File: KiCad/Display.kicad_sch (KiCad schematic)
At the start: 36 parts, among them J1 DC, J2 I/O, J3 USB-C, U1 ESP32-PICO-MINI-02, U2 L96-M33, U3 FT231XQ, U4 LMR16006+FB, U5 QR

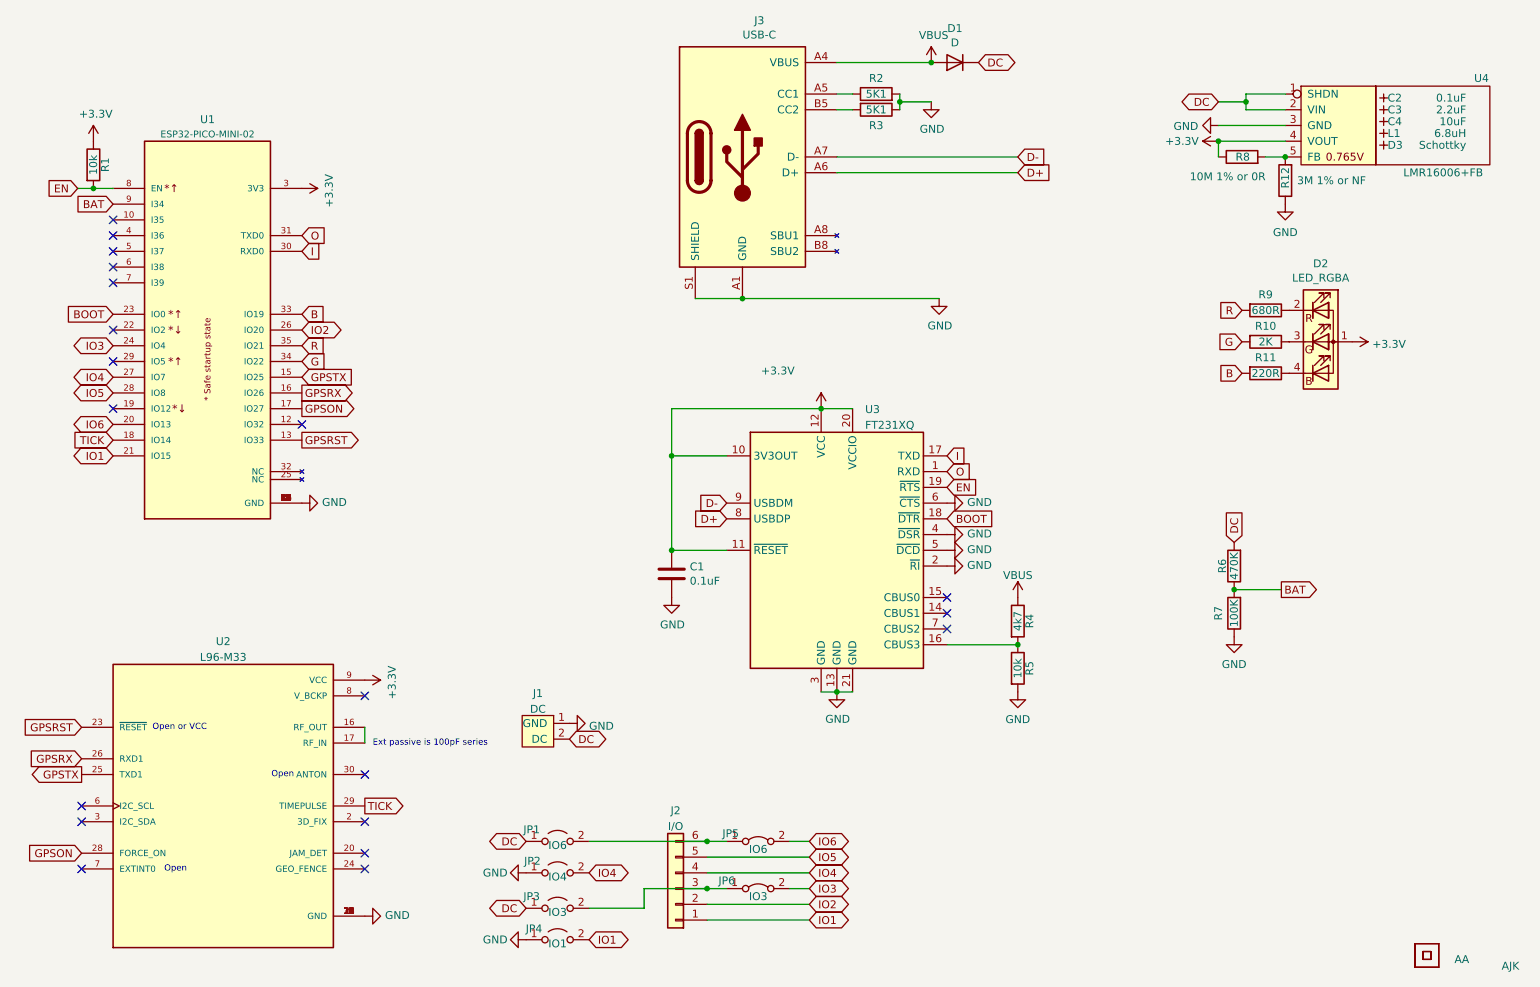
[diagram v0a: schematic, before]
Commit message: Started on Display board.
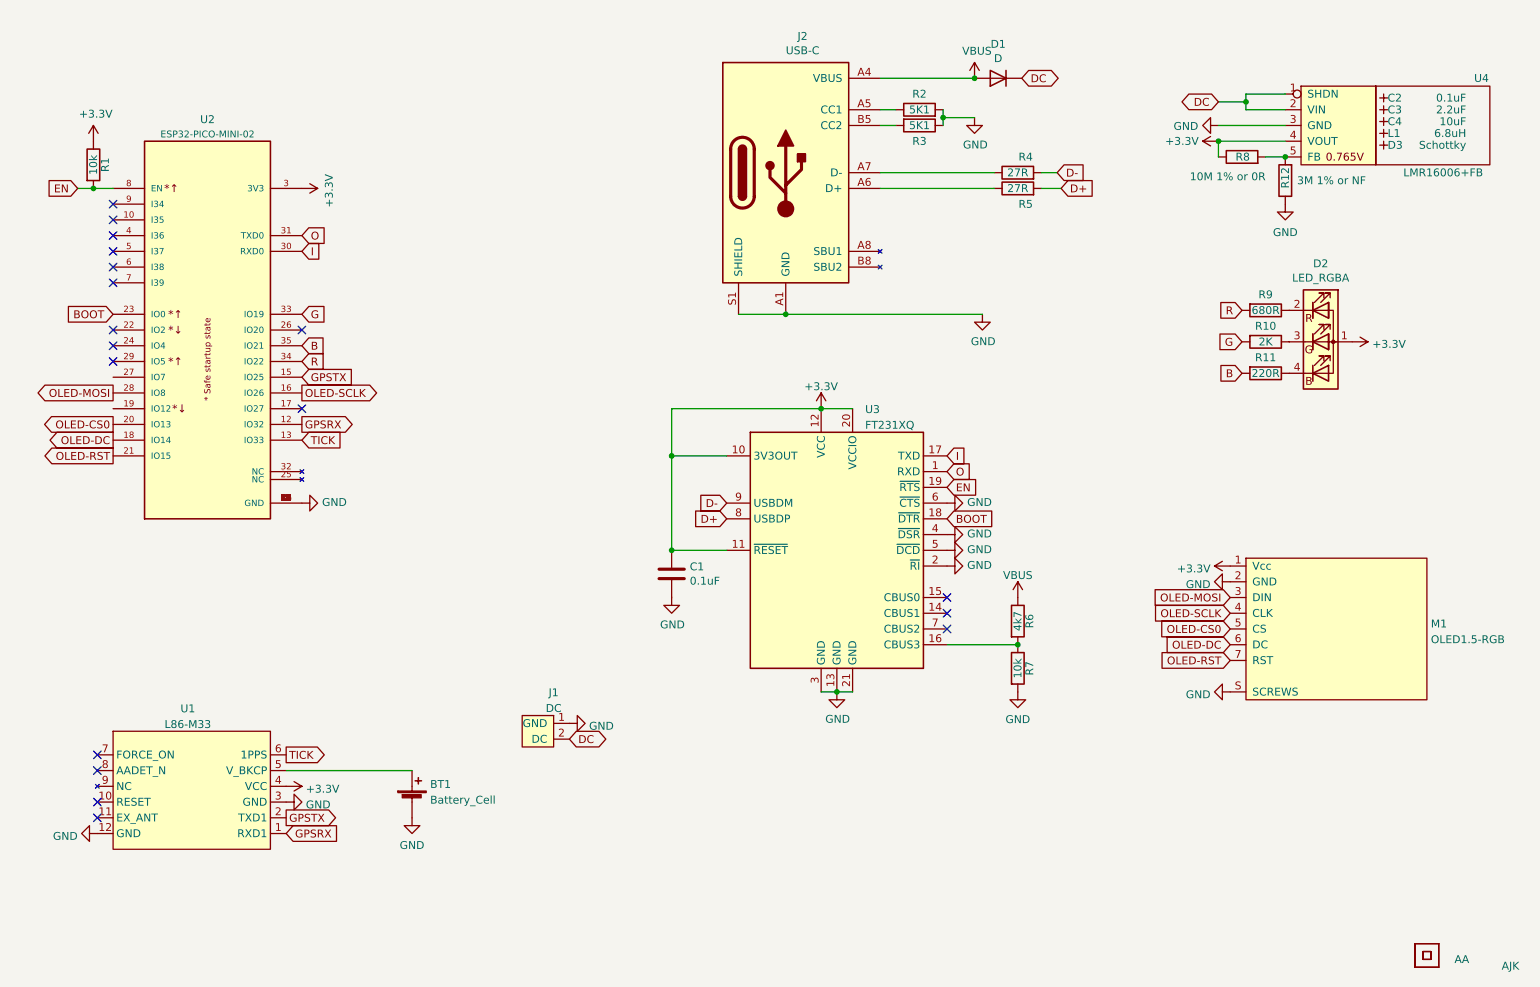
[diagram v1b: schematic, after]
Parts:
- removed J2: I/O, RevK:Molex_MiniSPOX_H6RA, symbol Connector_Generic:Conn_01x06
- removed JP1: IO6, RevK:Pad_1206_0805_Open, symbol Jumper:Jumper_2_Open
- removed JP2: IO4, RevK:Pad_1206_0805_Open, symbol Jumper:Jumper_2_Open
- removed JP3: IO3, RevK:Pad_1206_0805_Open, symbol Jumper:Jumper_2_Open
- removed JP4: IO1, RevK:Pad_1206_0805_Open, symbol Jumper:Jumper_2_Open
- removed JP5: IO6, RevK:Pad_1206_0805_Bridged, symbol Jumper:Jumper_2_Bridged
- removed JP6: IO3, RevK:Pad_1206_0805_Bridged, symbol Jumper:Jumper_2_Bridged
- removed R6: 470K, RevK:R_0603, symbol Device:R
- removed R7: 100K, RevK:R_0603, symbol Device:R
- removed U2: L96-M33, RevK:L96-M33, symbol RevK:L96-M33
- added BT1: Battery_Cell, Battery:BatteryHolder_Keystone_3002_1x2032, symbol Device:Battery_Cell
- added M1: OLED1.5-RGB, RevK:OLED1.5-RGB, symbol RevK:OLED1.5-RGB
- added R4, R5: 27R, RevK:R_0603, symbol Device:R
- added U1: L86-M33, RevK:L86-M33, symbol RevK:L86-M33
- renumbered J3 to J2, R4 to R6, R5 to R7, U1 to U2
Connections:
- net GPSRST is gone; now on net TICK: U2.13 (IO33)
- net +3V3: now also M1.1 (Vcc), U1.4 (VCC)
- net B: now also U2.35 (IO21); no longer U2.33 (IO19)
- net D+: now also R5.2; no longer J2.A6 (D+), J2.B6 (D+)
- net D-: now also R4.2; no longer J2.A7 (D-), J2.B7 (D-)
- net G: now also U2.33 (IO19); no longer U2.34 (IO22)
- net GND: now also BT1.2 (-), M1.2 (GND), M1.S (SCREWS), U1.12 (GND), U1.3 (GND)
- net GPSRX: now also U2.12 (IO32), U1.1 (RXD1); no longer U2.16 (IO26)
- net GPSTX: now also U1.2 (TXD1)
- net R: now also U2.34 (IO22); no longer U2.35 (IO21)
- net TICK: now also U1.6 (1PPS); no longer U2.18 (IO14)
- net BAT: no longer names the net of U2.9 (I34)
- net GPSON: no longer names the net of U2.17 (IO27)
- net IO1 renamed OLED-RST
- net OLED-RST: now also M1.7 (RST)
- net IO2: no longer names the net of U2.26 (IO20)
- net IO3: no longer names the net of U2.24 (IO4)
- net IO4: no longer names the net of U2.27 (IO7)
- net IO5 renamed OLED-MOSI
- net OLED-MOSI: now also M1.3 (DIN)
- net IO6 renamed OLED-CS0
- net OLED-CS0: now also M1.5 (CS)
- new net: J2.A6 (D+), J2.B6 (D+), R5.1
- new net: J2.A7 (D-), J2.B7 (D-), R4.1
- new net: BT1.1 (+), U1.5 (V_BKCP)
- new net OLED-DC: M1.6 (DC), U2.18 (IO14)
- new net OLED-SCLK: M1.4 (CLK), U2.16 (IO26)
- no-connect marks 20 -> 18
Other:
- note removed: "Ext passive is 100pF series"
- note removed: "Open"
- note removed: "Open or VCC"
- title: GPS / Glider control board -> GPS reference
- moved on the sheet: D1, J2, R2, R3
